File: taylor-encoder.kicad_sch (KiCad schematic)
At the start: 0 parts

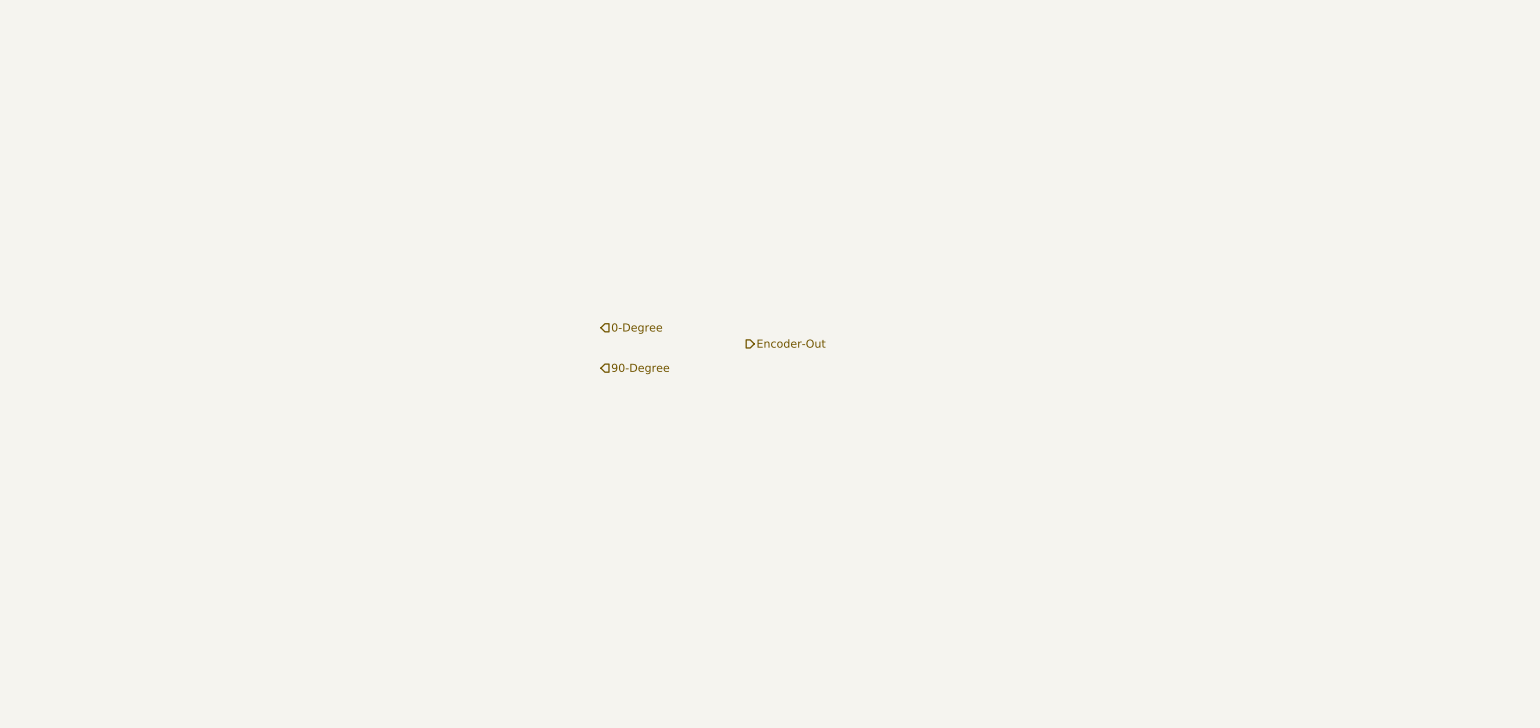
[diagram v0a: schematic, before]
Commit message: lots of updates
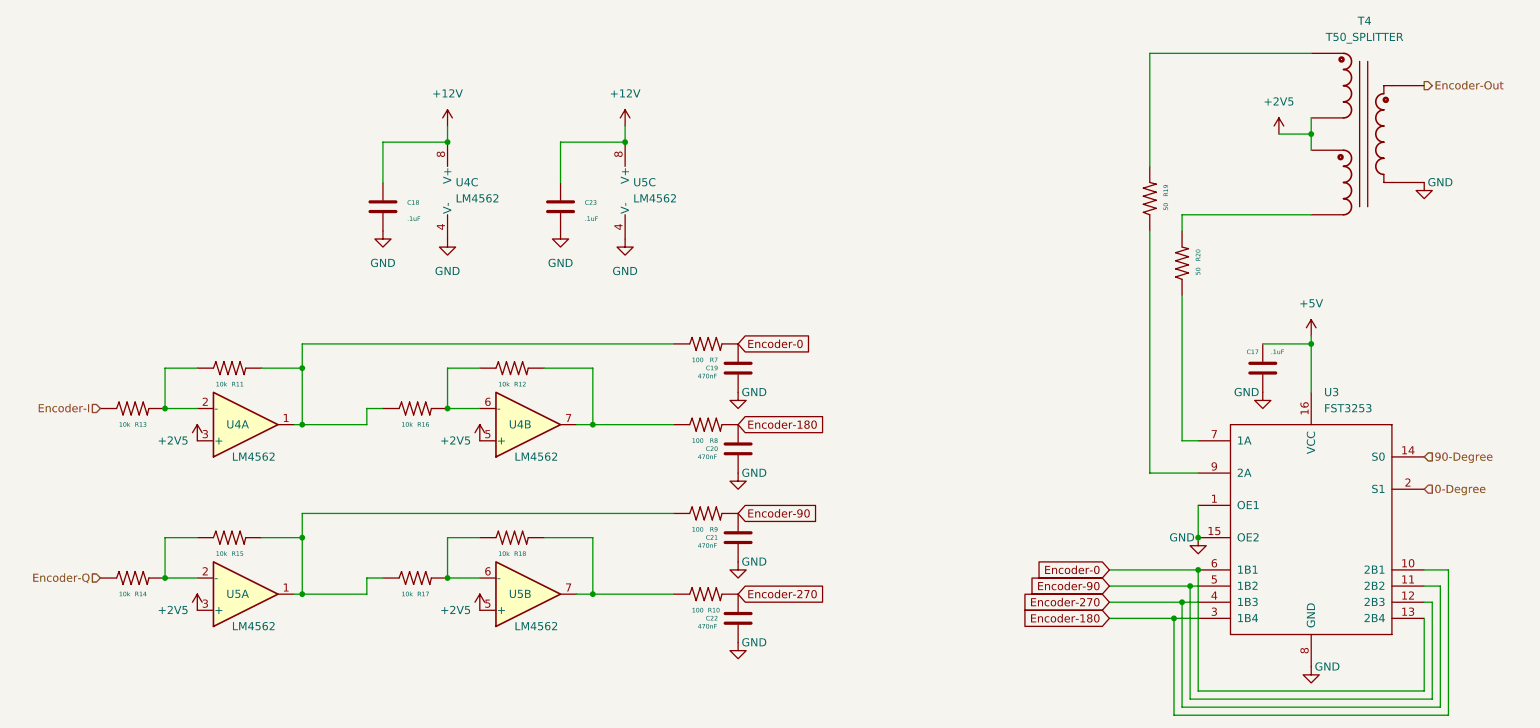
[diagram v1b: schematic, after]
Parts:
- added C17, C18, C23: .1uF, Capacitor_SMD:C_1206_3216Metric, symbol Xenir:Capacitor
- added C19, C20, C21, C22: 470nF, Capacitor_SMD:C_1206_3216Metric, symbol Xenir:Capacitor
- added R10, R7, R8, R9: 100, Resistor_SMD:R_0805_2012Metric, symbol Xenir:Resistor
- added R11, R12, R13, R14, R15, R16, R17, R18: 10k, Resistor_SMD:R_0805_2012Metric, symbol Xenir:Resistor
- added R19, R20: 50, Resistor_SMD:R_0805_2012Metric, symbol Xenir:Resistor
- added T4: T50_SPLITTER, Xenir:T50 Trifilar, symbol Xenir:T50_SPLITTER
- added U3: FST3253, Xenir:SO16, symbol Xenir:FST3253
- added U4, U5: LM4562, Xenir:SO08, symbol Amplifier_Operational:LM358
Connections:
- net 0-Degree: now also U3.2 (S1)
- net 90-Degree: now also U3.14 (S0)
- net Encoder-Out: now also T4.C1B
- new net: R14.2, R15.1, U5.2 (-)
- new net: R15.2, R17.1, R9.1, U5.1
- new net: R11.2, R16.1, R7.1, U4.1
- new net: R20.1, U3.7 (1A)
- new net: R19.1, U3.9 (2A)
- new net: R19.2, T4.C2B
- new net: R20.2, T4.C3A
- new net: R12.1, R16.2, U4.6 (-)
- new net: R12.2, R8.1, U4.7
- new net: R11.1, R13.2, U4.2 (-)
- new net: R17.2, R18.1, U5.6 (-)
- new net: R10.1, R18.2, U5.7
- new net +12V: C18.2, C23.2, U4.8 (V+), U5.8 (V+)
- new net +2V5: T4.C2A, T4.C3B, U4.3 (+), U4.5 (+), U5.3 (+), U5.5 (+)
- new net +5V: C17.2, U3.16 (VCC)
- new net Encoder-0: C19.2, R7.2, U3.13 (2B4), U3.6 (1B1)
- new net Encoder-180: C20.2, R8.2, U3.10 (2B1), U3.3 (1B4)
- new net Encoder-270: C22.2, R10.2, U3.11 (2B2), U3.4 (1B3)
- new net Encoder-90: C21.2, R9.2, U3.12 (2B3), U3.5 (1B2)
- new net Encoder-I: R13.1
- new net Encoder-Q: R14.1
- new net GND: C17.1, C18.1, C19.1, C20.1, C21.1, C22.1, C23.1, T4.C1A, U3.1 (OE1), U3.15 (OE2), U3.8 (GND), U4.4 (V-), U5.4 (V-)
